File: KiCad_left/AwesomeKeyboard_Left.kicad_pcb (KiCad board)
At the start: 2 copper layers, 140 x 109 mm, 57 parts, among them J1 AudioJack4_Ground, SW1 SW_DIP_x01, SW11 SW_Push, SW12 SW_Push, SW13 SW_Push, SW14 SW_Push, SW15 SW_Push, SW16 SW_Push, SW21 SW_Push, SW22 SW_Push, SW23 SW_Push, SW24 SW_Push, SW25 SW_Push, SW26 SW_Push, SW31 SW_Push, SW32 SW_Push, SW33 SW_Push, SW34 SW_Push, SW35 SW_Push, SW36 SW_Push, SW45 SW_Push, SW46 SW_Push

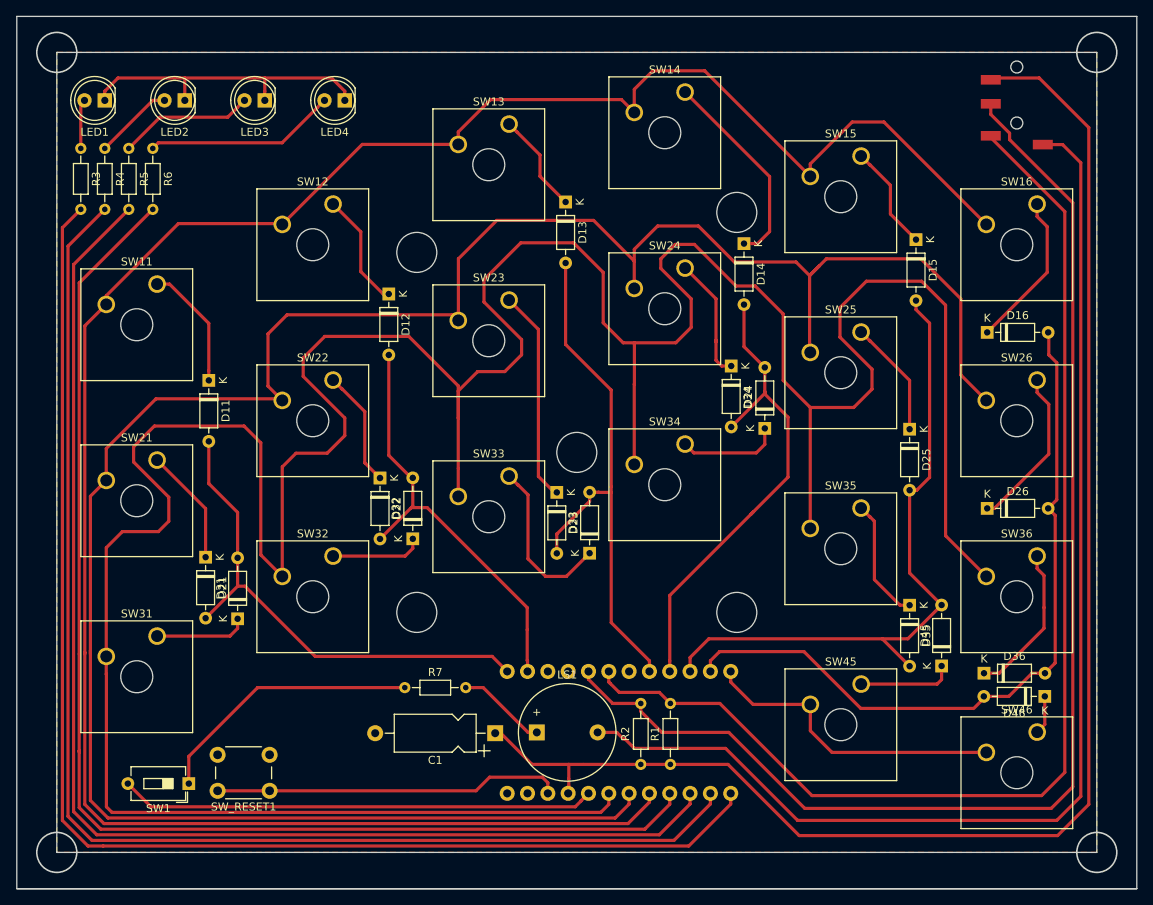
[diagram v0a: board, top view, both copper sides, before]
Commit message: left
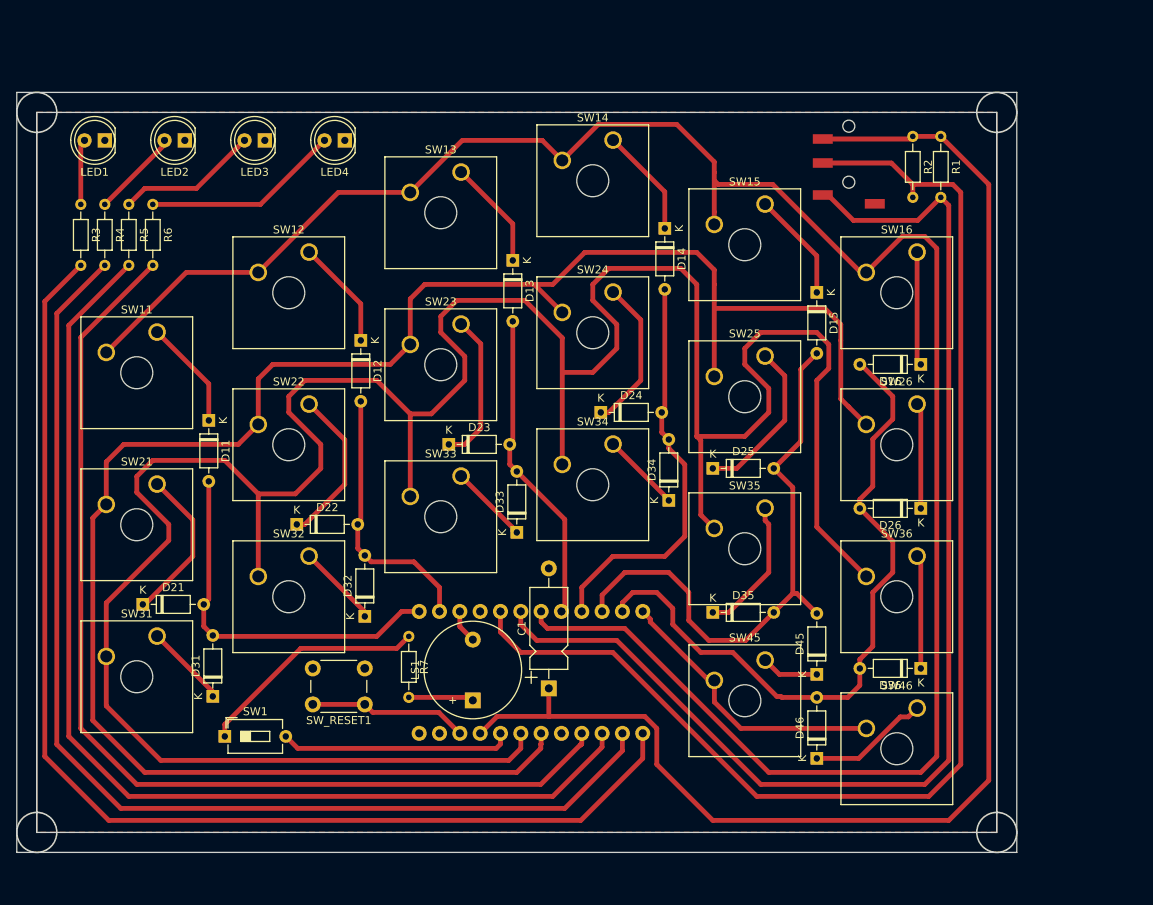
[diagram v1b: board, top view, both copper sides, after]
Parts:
- moved R2 85.5 mm to (184.8, 85.2), turned to 270 degrees
- moved R1 85.5 mm to (188.3, 85.2), turned to 270 degrees
- moved D46 29.5 mm to (172.8, 162.9), turned to 90 degrees
- moved D25 25.1 mm to (159.8, 126.7), turned to 0 degrees
- moved D35 24.6 mm to (159.8, 144.7), turned to 0 degrees
- moved J1 22.3 mm to (176.8, 88.7)
- moved D24 17.3 mm to (145.8, 119.7), turned to 0 degrees
- moved SW16 16.2 mm to (185.3, 99.6)
- moved SW_RESET1 16.1 mm to (116.3, 156.2)
- moved D45 15.6 mm to (172.8, 152.4)
- moved SW26 15.3 mm to (185.3, 118.6)
- moved SW46 15.3 mm to (185.3, 156.6)
- moved SW36 15.0 mm to (185.3, 137.6)
- moved D34 15.0 mm to (154.3, 130.7)
- moved D23 14.8 mm to (126.8, 123.7), turned to 0 degrees
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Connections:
- B1 pad 17: /ROW1 -> (no net)
- B1 pad 23: Net-(B1-Pad23) -> (no net)
- B1 pad 24: Net-(B1-Pad24) -> (no net)
- B1 pad 4: Net-(B1-Pad4) -> (no net)
- B1 pad 7: Net-(B1-Pad7) -> /ROW1
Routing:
- net GND: track 190.4 -> 4.19 mm
- net /ROW3: track 432.7 -> 345.2 mm
- net /ROW2: track 285.7 -> 238.0 mm
- net /SPEAKER: track 59.5 -> 29.0 mm
- net /COL3: track 67.7 -> 39.4 mm
- net /LED4: track 156.4 -> 130.5 mm
- net Net-(B1-Pad22): track 43.6 -> 19.9 mm
- net /LED3: track 159.3 -> 136.0 mm
- net /ROW1: track 278.8 -> 257.6 mm
- net /LED2: track 162.5 -> 141.5 mm
- net /COL2: track 53.8 -> 33.8 mm
- net /LED1: track 165.7 -> 147.6 mm
- net /COL1: track 63.4 -> 47.1 mm
- net Net-(D14-Pad1): track 25.6 -> 13.7 mm
- net Net-(D33-Pad1): track 21.1 -> 10.5 mm
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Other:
- board size 140 x 109 mm -> 125 x 95 mm
- net class Default: trace_width 0.4 -> 0.6
